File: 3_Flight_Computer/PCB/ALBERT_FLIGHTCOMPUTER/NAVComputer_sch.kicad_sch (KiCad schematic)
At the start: 25 parts, among them J1 USB_B_Micro, J2 Conn_01x05, SW1 SW_SPDT, Y1 16MHz

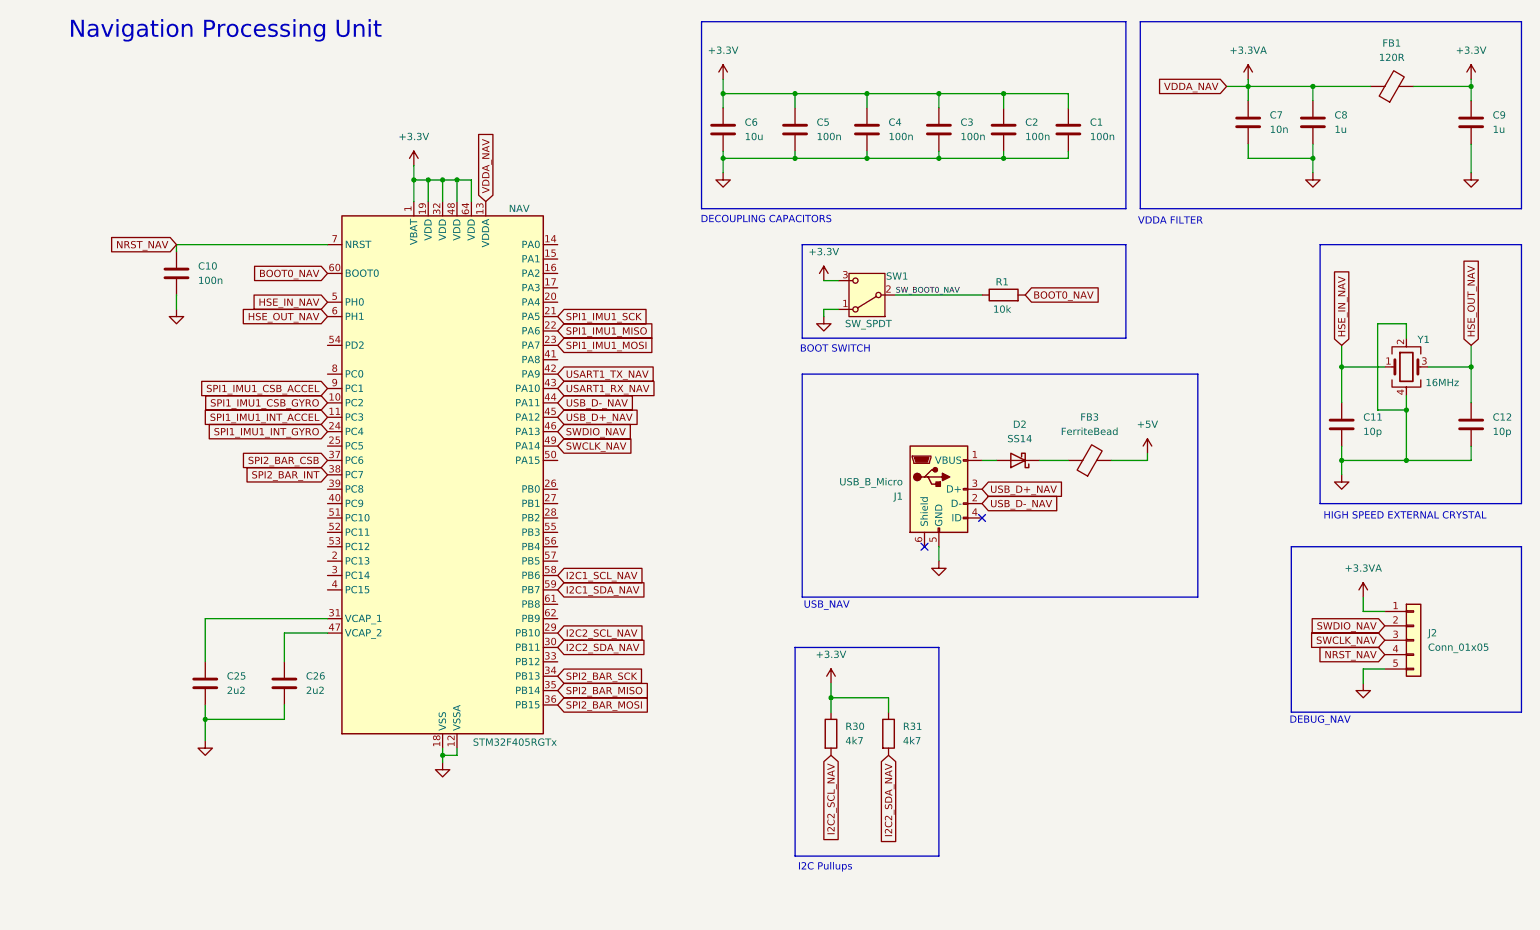
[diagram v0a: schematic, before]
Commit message: Refactor code structure for improved readability and maintainability
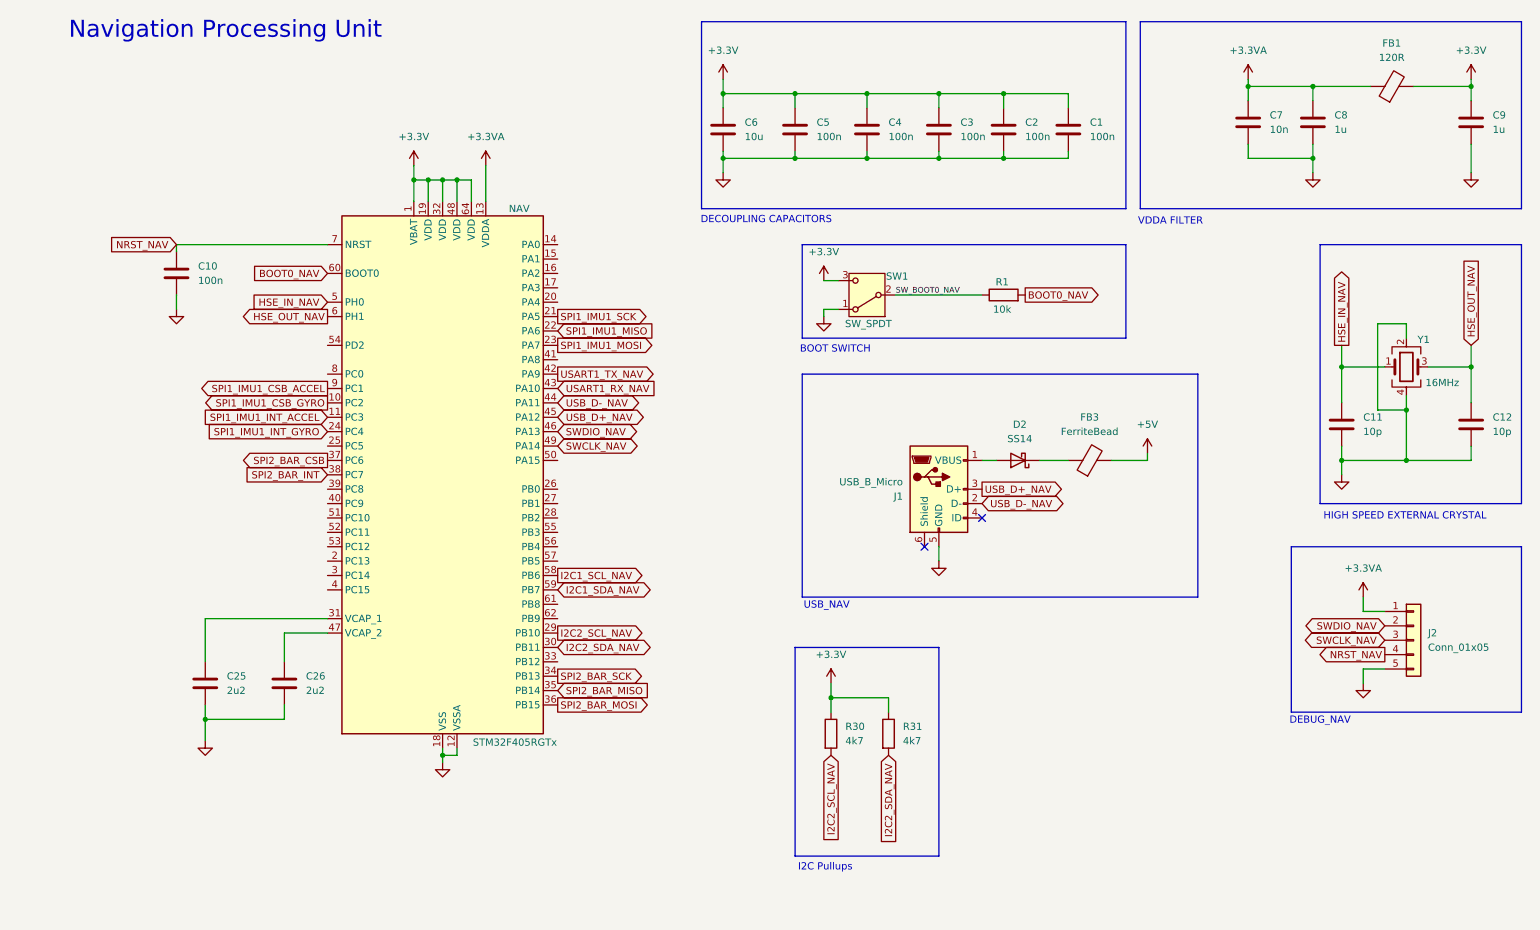
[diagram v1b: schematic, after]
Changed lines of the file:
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@@
 	(wire
 		(pts
+			(xy 92.71 41.91) (xy 92.71 48.26)
+		)
+		(stroke
+			(width 0)
+			(type default)
+		)
+	)
+	(wire
+		(pts
 			(xy 247.65 130.81) (xy 251.46 130.81)
 		)
@@
 	(wire
 		(pts
-			(xy 223.52 27.94) (xy 227.33 27.94)
-		)
-		(stroke
-			(width 0)
-			(type default)
-		)
-	)
-	(wire
-		(pts
 			(xy 266.7 27.94) (xy 266.7 30.48)
 		)
@@
 	)
 	(global_label "I2C2_SCL_NAV"
-		(shape input)
+		(shape output)
 		(at 105.41 124.46 0)
 		(fields_autoplaced yes)
@@
 	)
 	(global_label "I2C2_SDA_NAV"
-		(shape input)
+		(shape bidirectional)
 		(at 105.41 127 0)
 		(fields_autoplaced yes)
@@
 		)
 		(property "Intersheetrefs" "${INTERSHEET_REFS}"
-			(at 121.7 127 0)
+			(at 122.8113 127 0)
 			(effects
 				(font
@@
 	)
 	(global_label "SPI1_IMU1_CSB_ACCEL"
-		(shape input)
+		(shape output)
 		(at 64.77 81.28 180)
 		(fields_autoplaced yes)
@@
 	)
 	(global_label "USB_D-_NAV"
-		(shape input)
+		(shape bidirectional)
 		(at 105.41 83.82 0)
 		(fields_autoplaced yes)
@@
 		)
 		(property "Intersheetrefs" "${INTERSHEET_REFS}"
-			(at 120.4905 83.82 0)
+			(at 121.6018 83.82 0)
 			(effects
 				(font
@@
 	)
 	(global_label "BOOT0_NAV"
-		(shape input)
+		(shape output)
 		(at 187.96 64.77 0)
 		(fields_autoplaced yes)
@@
 	)
 	(global_label "SWCLK_NAV"
-		(shape input)
+		(shape bidirectional)
 		(at 251.46 125.73 180)
 		(fields_autoplaced yes)
@@
 		)
 		(property "Intersheetrefs" "${INTERSHEET_REFS}"
-			(at 237.7705 125.73 0)
+			(at 236.6592 125.73 0)
 			(effects
 				(font
@@
 	)
 	(global_label "SWDIO_NAV"
-		(shape input)
+		(shape bidirectional)
 		(at 105.41 88.9 0)
 		(fields_autoplaced yes)
@@
 		)
 		(property "Intersheetrefs" "${INTERSHEET_REFS}"
-			(at 118.7367 88.9 0)
+			(at 119.848 88.9 0)
 			(effects
 				(font
@@
 	)
 	(global_label "HSE_IN_NAV"
-		(shape input)
+		(shape output)
 		(at 243.84 73.66 90)
 		(fields_autoplaced yes)
@@
 	)
 	(global_label "SWDIO_NAV"
-		(shape input)
+		(shape bidirectional)
 		(at 251.46 123.19 180)
 		(fields_autoplaced yes)
@@
 		)
 		(property "Intersheetrefs" "${INTERSHEET_REFS}"
-			(at 238.1333 123.19 0)
+			(at 237.022 123.19 0)
 			(effects
 				(font
@@
 	)
 	(global_label "HSE_OUT_NAV"
-		(shape input)
+		(shape output)
 		(at 64.77 68.58 180)
 		(fields_autoplaced yes)
@@
 	)
 	(global_label "SPI1_IMU1_SCK"
-		(shape input)
+		(shape output)
 		(at 105.41 68.58 0)
 		(fields_autoplaced yes)
@@
 	)
 	(global_label "NRST_NAV"
-		(shape input)
+		(shape output)
 		(at 251.46 128.27 180)
 		(fields_autoplaced yes)
@@
 	)
 	(global_label "I2C1_SDA_NAV"
-		(shape input)
+		(shape bidirectional)
 		(at 105.41 116.84 0)
 		(fields_autoplaced yes)
@@
 		)
 		(property "Intersheetrefs" "${INTERSHEET_REFS}"
-			(at 121.7 116.84 0)
+			(at 122.8113 116.84 0)
 			(effects
 				(font
@@
 	)
 	(global_label "I2C1_SCL_NAV"
-		(shape input)
+		(shape output)
 		(at 105.41 114.3 0)
 		(fields_autoplaced yes)
@@
 	)
 	(global_label "SPI2_BAR_MOSI"
-		(shape input)
+		(shape output)
 		(at 105.41 137.16 0)
 		(fields_autoplaced yes)
@@
 	)
 	(global_label "USB_D+_NAV"
-		(shape input)
+		(shape bidirectional)
 		(at 105.41 86.36 0)
 		(fields_autoplaced yes)
@@
 		)
 		(property "Intersheetrefs" "${INTERSHEET_REFS}"
-			(at 120.4905 86.36 0)
+			(at 121.6018 86.36 0)
 			(effects
 				(font
@@
 	)
 	(global_label "SPI2_BAR_SCK"
-		(shape input)
+		(shape output)
 		(at 105.41 132.08 0)
 		(fields_autoplaced yes)
@@
 	)
 	(global_label "USB_D+_NAV"
-		(shape input)
+		(shape output)
 		(at 180.34 99.06 0)
 		(fields_autoplaced yes)
@@
 		)
 	)
-	(global_label "VDDA_NAV"
-		(shape input)
-		(at 92.71 48.26 90)
-		(fields_autoplaced yes)
-		(effects
-			(font
-				(size 1.27 1.27)
-			)
-			(justify left)
-		)
-		(property "Intersheetrefs" "${INTERSHEET_REFS}"
-			(at 92.71 36.0823 90)
-			(effects
-				(font
-					(size 1.27 1.27)
-				)
-				(justify left)
-				(hide yes)
-			)
-		)
-	)
 	(global_label "USART1_TX_NAV"
-		(shape input)
+		(shape output)
 		(at 105.41 78.74 0)
 		(fields_autoplaced yes)
@@
 	)
 	(global_label "USB_D-_NAV"
-		(shape input)
+		(shape bidirectional)
 		(at 180.34 101.6 0)
 		(fields_autoplaced yes)
@@
 		)
 		(property "Intersheetrefs" "${INTERSHEET_REFS}"
-			(at 195.4205 101.6 0)
+			(at 196.5318 101.6 0)
 			(effects
 				(font
@@
 		)
 	)
-	(global_label "VDDA_NAV"
-		(shape input)
-		(at 223.52 27.94 180)
-		(fields_autoplaced yes)
-		(effects
-			(font
-				(size 1.27 1.27)
-			)
-			(justify right)
-		)
-		(property "Intersheetrefs" "${INTERSHEET_REFS}"
-			(at 211.3423 27.94 0)
-			(effects
-				(font
-					(size 1.27 1.27)
-				)
-				(justify right)
-				(hide yes)
-			)
-		)
-	)
 	(global_label "SWCLK_NAV"
-		(shape input)
+		(shape bidirectional)
 		(at 105.41 91.44 0)
 		(fields_autoplaced yes)
@@
 		)
 		(property "Intersheetrefs" "${INTERSHEET_REFS}"
-			(at 119.0995 91.44 0)
+			(at 120.2108 91.44 0)
 			(effects
 				(font
@@
 	)
 	(global_label "SPI1_IMU1_MOSI"
-		(shape input)
+		(shape output)
 		(at 105.41 73.66 0)
 		(fields_autoplaced yes)
@@
 	)
 	(global_label "SPI1_IMU1_CSB_GYRO"
-		(shape input)
+		(shape output)
 		(at 64.77 83.82 180)
 		(fields_autoplaced yes)
@@
 	)
 	(global_label "SPI2_BAR_CSB"
-		(shape input)
+		(shape output)
 		(at 64.77 93.98 180)
 		(fields_autoplaced yes)
@@
 					(unit 1)
 				)
+			)
+		)
+	)
+	(symbol
+		(lib_id "power:+3.3V")
+		(at 92.71 41.91 0)
+		(unit 1)
+		(exclude_from_sim no)
+		(in_bom yes)
+		(on_board yes)
+		(dnp no)
+		(fields_autoplaced yes)
+		(property "Reference" "#PWR093"
+			(at 92.71 45.72 0)
+			(effects
+				(font
+					(size 1.27 1.27)
+				)
+				(hide yes)
+			)
+		)
+		(property "Value" "+3.3VA"
+			(at 92.71 36.83 0)
+			(effects
+				(font
+					(size 1.27 1.27)
+				)
+			)
+		)
+		(property "Footprint" ""
+			(at 92.71 41.91 0)
+			(effects
+				(font
+					(size 1.27 1.27)
+				)
+				(hide yes)
+			)
+		)
+		(property "Datasheet" ""
+			(at 92.71 41.91 0)
+			(effects
+				(font
+					(size 1.27 1.27)
+				)
+				(hide yes)
+			)
+		)
+		(property "Description" "Power symbol creates a global label with name \"+3.3V\""
+			(at 92.71 41.91 0)
+			(effects
+				(font
+					(size 1.27 1.27)
+				)
+				(hide yes)
+			)
+		)
+		(pin "1"
+		)
+		(instances
+			(project "ALBERT_FLIGHTCOMPUTER"
+				(path "/caf1b85f-a91d-4c85-9df1-65f9ebc85027/7985d733-09dc-4902-a3ab-fbbf0df3c379"
+					(reference "#PWR093")
+					(unit 1)
+				)

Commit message: Add lock file for ALBERT_FLIGHTCOMPUTER PCB design
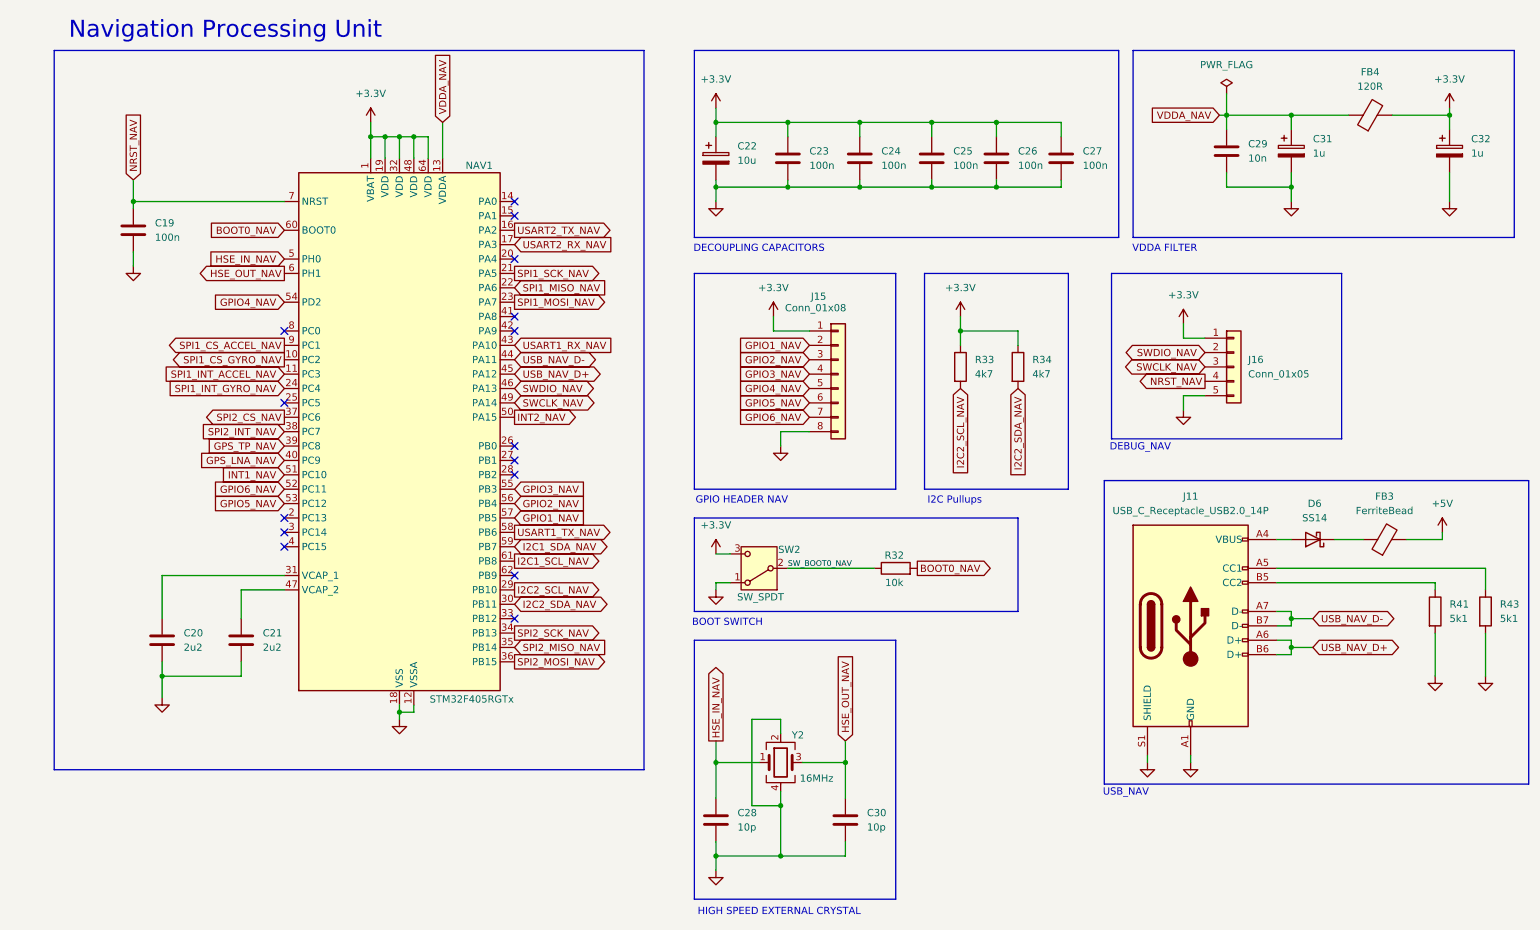
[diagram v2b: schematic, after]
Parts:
- removed C6: 10u, symbol Device:C
- removed C8, C9: 1u, symbol Device:C
- removed J1: USB_B_Micro, symbol Connector:USB_B_Micro
- added C22: 10u, Capacitor_Tantalum_SMD:CP_EIA-1608-10_AVX-L, symbol Device:C_Polarized
- added C31, C32: 1u, Capacitor_Tantalum_SMD:CP_EIA-1608-10_AVX-L, symbol Device:C_Polarized
- added J11: USB_C_Receptacle_USB2.0_14P, Connector_USB:USB_C_Receptacle_HRO_TYPE-C-31-M-12, symbol Connector:USB_C_Receptacle_USB2.0_14P
- added J15: Conn_01x08, Connector_PinHeader_2.54mm:PinHeader_1x08_P2.54mm_Vertical, symbol Connector_Generic:Conn_01x08
- added R41, R43: 5k1, Resistor_SMD:R_0402_1005Metric, symbol Device:R
- C19: renamed from C10; footprint (none) -> Capacitor_SMD:C_0402_1005Metric
- C20: renamed from C25; footprint (none) -> Capacitor_SMD:C_0805_2012Metric
- C21: renamed from C26; footprint (none) -> Capacitor_SMD:C_0805_2012Metric
- C23: renamed from C5; footprint (none) -> Capacitor_SMD:C_0402_1005Metric
- C24: renamed from C4; footprint (none) -> Capacitor_SMD:C_0402_1005Metric
- C25: renamed from C3; footprint (none) -> Capacitor_SMD:C_0402_1005Metric
- C26: renamed from C2; footprint (none) -> Capacitor_SMD:C_0402_1005Metric
- C27: renamed from C1; footprint (none) -> Capacitor_SMD:C_0402_1005Metric
- C28: renamed from C11; footprint (none) -> Capacitor_SMD:C_0402_1005Metric
- C29: renamed from C7; footprint (none) -> Capacitor_SMD:C_0402_1005Metric
- C30: renamed from C12; footprint (none) -> Capacitor_SMD:C_0402_1005Metric
- FB3: footprint (none) -> Inductor_SMD:L_0603_1608Metric
- FB4: renamed from FB1; footprint (none) -> Inductor_SMD:L_0603_1608Metric
- J16: renamed from J2; footprint (none) -> Connector_PinHeader_2.54mm:PinHeader_1x05_P2.54mm_Vertical
- R32: renamed from R1; footprint (none) -> Resistor_SMD:R_0402_1005Metric
- R33: renamed from R30; footprint (none) -> Resistor_SMD:R_0402_1005Metric
- R34: renamed from R31; footprint (none) -> Resistor_SMD:R_0402_1005Metric
- SW2: renamed from SW1; footprint (none) -> Button_Switch_SMD:SW_SPDT_PCM12
- Y2: renamed from Y1; footprint (none) -> Crystal:Crystal_SMD_3225-4Pin_3.2x2.5mm
- renumbered D2 to D6, NAV to NAV1
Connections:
- net +3.3V: now also J16.1 (Pin_1), C22.1, C32.1, J15.1 (Pin_1)
- net GND: now also C22.2, C31.2, C32.2, J11.A1 (GND), J11.A12 (GND), J11.B1 (GND), J11.B12 (GND), J11.S1 (SHIELD), J15.8 (Pin_8), R41.2, R43.2
- net I2C1_SCL_NAV: now also NAV1.61 (PB8); no longer NAV1.58 (PB6)
- net USART1_TX_NAV: now also NAV1.58 (PB6); no longer NAV1.42 (PA9)
- net USART2_TX_NAV: now reaches NAV1.16 (PA2)
- net USART2_RX_NAV: now reaches NAV1.17 (PA3)
- net GPS_TP_NAV: now reaches NAV1.39 (PC8)
- net GPS_LNA_NAV: now reaches NAV1.40 (PC9)
- net INT2_NAV: now reaches NAV1.50 (PA15)
- net INT1_NAV: now reaches NAV1.51 (PC10)
- net GPIO6_NAV: now reaches NAV1.52 (PC11)
- net GPIO6_NAV: now also J15.7 (Pin_7)
- net GPIO5_NAV: now reaches NAV1.53 (PC12)
- net GPIO5_NAV: now also J15.6 (Pin_6)
- net GPIO4_NAV: now reaches NAV1.54 (PD2)
- net GPIO4_NAV: now also J15.5 (Pin_5)
- net GPIO3_NAV: now reaches NAV1.55 (PB3)
- net GPIO3_NAV: now also J15.4 (Pin_4)
- net GPIO2_NAV: now reaches NAV1.56 (PB4)
- net GPIO2_NAV: now also J15.3 (Pin_3)
- net GPIO1_NAV: now reaches NAV1.57 (PB5)
- net GPIO1_NAV: now also J15.2 (Pin_2)
- net at D6.2 (A): now also J11.A4 (VBUS), J11.A9 (VBUS), J11.B4 (VBUS), J11.B9 (VBUS)
- net +3.3VA renamed VDDA_NAV
- net VDDA_NAV: now also C31.1; no longer J16.1 (Pin_1)
- net SPI1_IMU1_CSB_ACCEL renamed SPI1_CS_ACCEL_NAV
- net SPI1_IMU1_CSB_GYRO renamed SPI1_CS_GYRO_NAV
- net SPI1_IMU1_INT_ACCEL renamed SPI1_INT_ACCEL_NAV
- net SPI1_IMU1_INT_GYRO renamed SPI1_INT_GYRO_NAV
- net SPI1_IMU1_MISO renamed SPI1_MISO_NAV
- net SPI1_IMU1_MOSI renamed SPI1_MOSI_NAV
- net SPI1_IMU1_SCK renamed SPI1_SCK_NAV
- net SPI2_BAR_CSB renamed SPI2_CS_NAV
- net SPI2_BAR_INT renamed SPI2_INT_NAV
- net SPI2_BAR_MISO renamed SPI2_MISO_NAV
- net SPI2_BAR_MOSI renamed SPI2_MOSI_NAV
- net SPI2_BAR_SCK renamed SPI2_SCK_NAV
- net USB_D+_NAV renamed USB_NAV_D+
- net USB_NAV_D+: now also J11.A6 (D+), J11.B6 (D+)
- net USB_D-_NAV renamed USB_NAV_D-
- net USB_NAV_D-: now also J11.A7 (D-), J11.B7 (D-)
- new net: J11.A5 (CC1), R43.1
- new net: J11.B5 (CC2), R41.1
- no-connect marks 2 -> 15
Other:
- note added: "GPIO HEADER NAV"
- company: (none) -> ALBERT AEROSPACE
- moved on the sheet: C19, C20, C21, C23, C24, C25, C26, C27, C28, C29, C30, D6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
